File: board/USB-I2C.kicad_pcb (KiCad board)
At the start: 2 copper layers, 44 x 18 mm, 17 parts, among them J1 USB_OTG, J2 Conn_01x06, U1 SPX3819, U2 STM32F042K4Tx, X1 I2C-6P, X2 I2C, X3 SWD

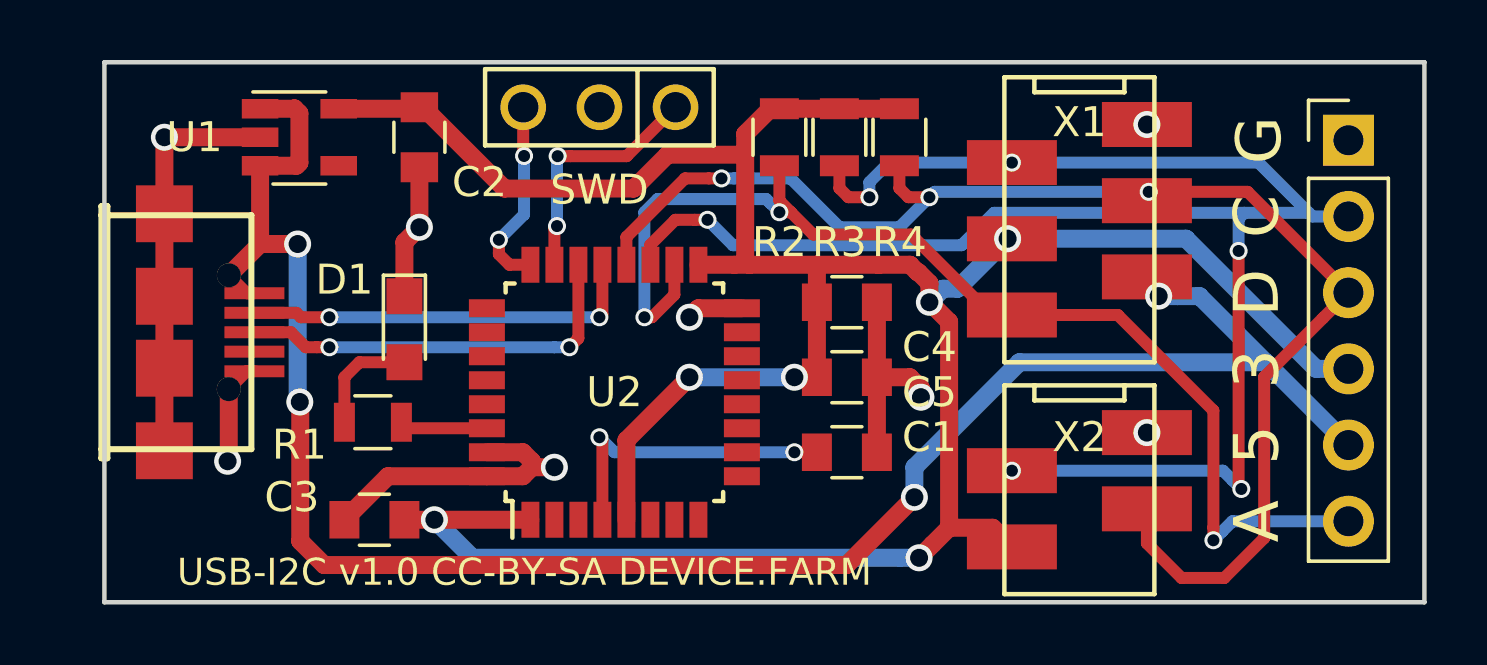
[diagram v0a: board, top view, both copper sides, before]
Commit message: WIP
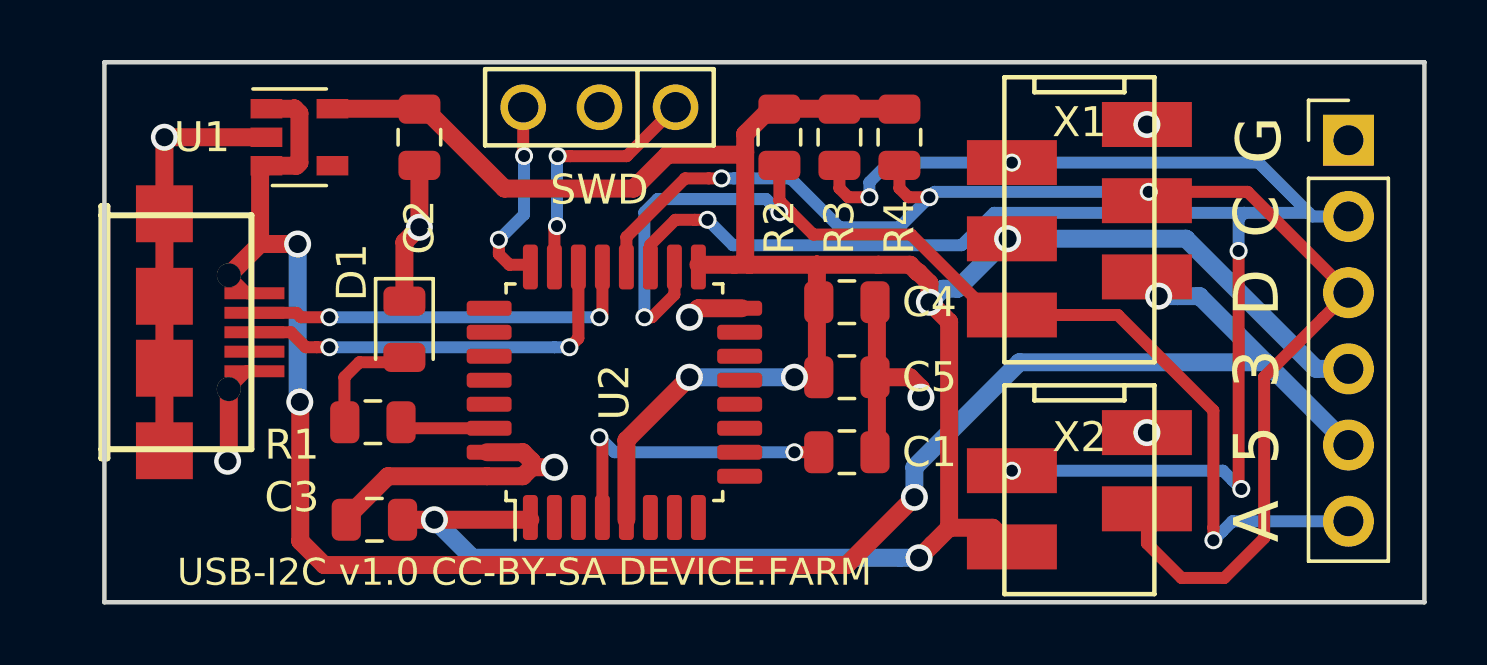
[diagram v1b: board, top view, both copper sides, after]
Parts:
- C1, C2, C3, C4, C5: footprint Capacitors_SMD:C_0805 -> Capacitor_SMD:C_0805_2012Metric
- D1: footprint LEDs:LED_0805 -> LED_SMD:LED_0805_2012Metric
- J2: footprint Pin_Headers:Pin_Header_Straight_1x06_Pitch2.54mm -> Connector_PinHeader_2.54mm:PinHeader_1x06_P2.54mm_Vertical
- R1, R2, R3, R4: footprint Resistors_SMD:R_0805 -> Resistor_SMD:R_0805_2012Metric
- U1: footprint TO_SOT_Packages_SMD:TSOT-23-5 -> Package_TO_SOT_SMD:SOT-23-5
- U2: footprint Housings_QFP:LQFP-32_7x7mm_Pitch0.8mm -> Package_QFP:LQFP-32_7x7mm_P0.8mm
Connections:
- J1 pad 4: (no net) -> Net-(J1-Pad4)
- U1 pad 4: (no net) -> Net-(U1-Pad4)
- U2 pad 10: (no net) -> Net-(U2-Pad10)
- U2 pad 11: (no net) -> Net-(U2-Pad11)
- U2 pad 12: (no net) -> Net-(U2-Pad12)
- U2 pad 13: (no net) -> Net-(U2-Pad13)
- U2 pad 14: (no net) -> Net-(U2-Pad14)
- U2 pad 15: (no net) -> Net-(U2-Pad15)
- U2 pad 2: (no net) -> Net-(U2-Pad2)
- U2 pad 25: (no net) -> Net-(U2-Pad25)
- U2 pad 26: (no net) -> Net-(U2-Pad26)
- U2 pad 27: (no net) -> Net-(U2-Pad27)
- U2 pad 28: (no net) -> Net-(U2-Pad28)
- U2 pad 29: (no net) -> Net-(U2-Pad29)
- U2 pad 3: (no net) -> Net-(U2-Pad3)
- U2 pad 6: (no net) -> Net-(U2-Pad6)
- U2 pad 7: (no net) -> Net-(U2-Pad7)
- U2 pad 8: (no net) -> Net-(U2-Pad8)
- U2 pad 9: (no net) -> Net-(U2-Pad9)
